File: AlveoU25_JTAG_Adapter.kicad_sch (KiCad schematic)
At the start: 11 parts, among them J1 Xilinx_JTAG, J3 OTHER, J4 OTHER, U1 Alveo_U25_Debug

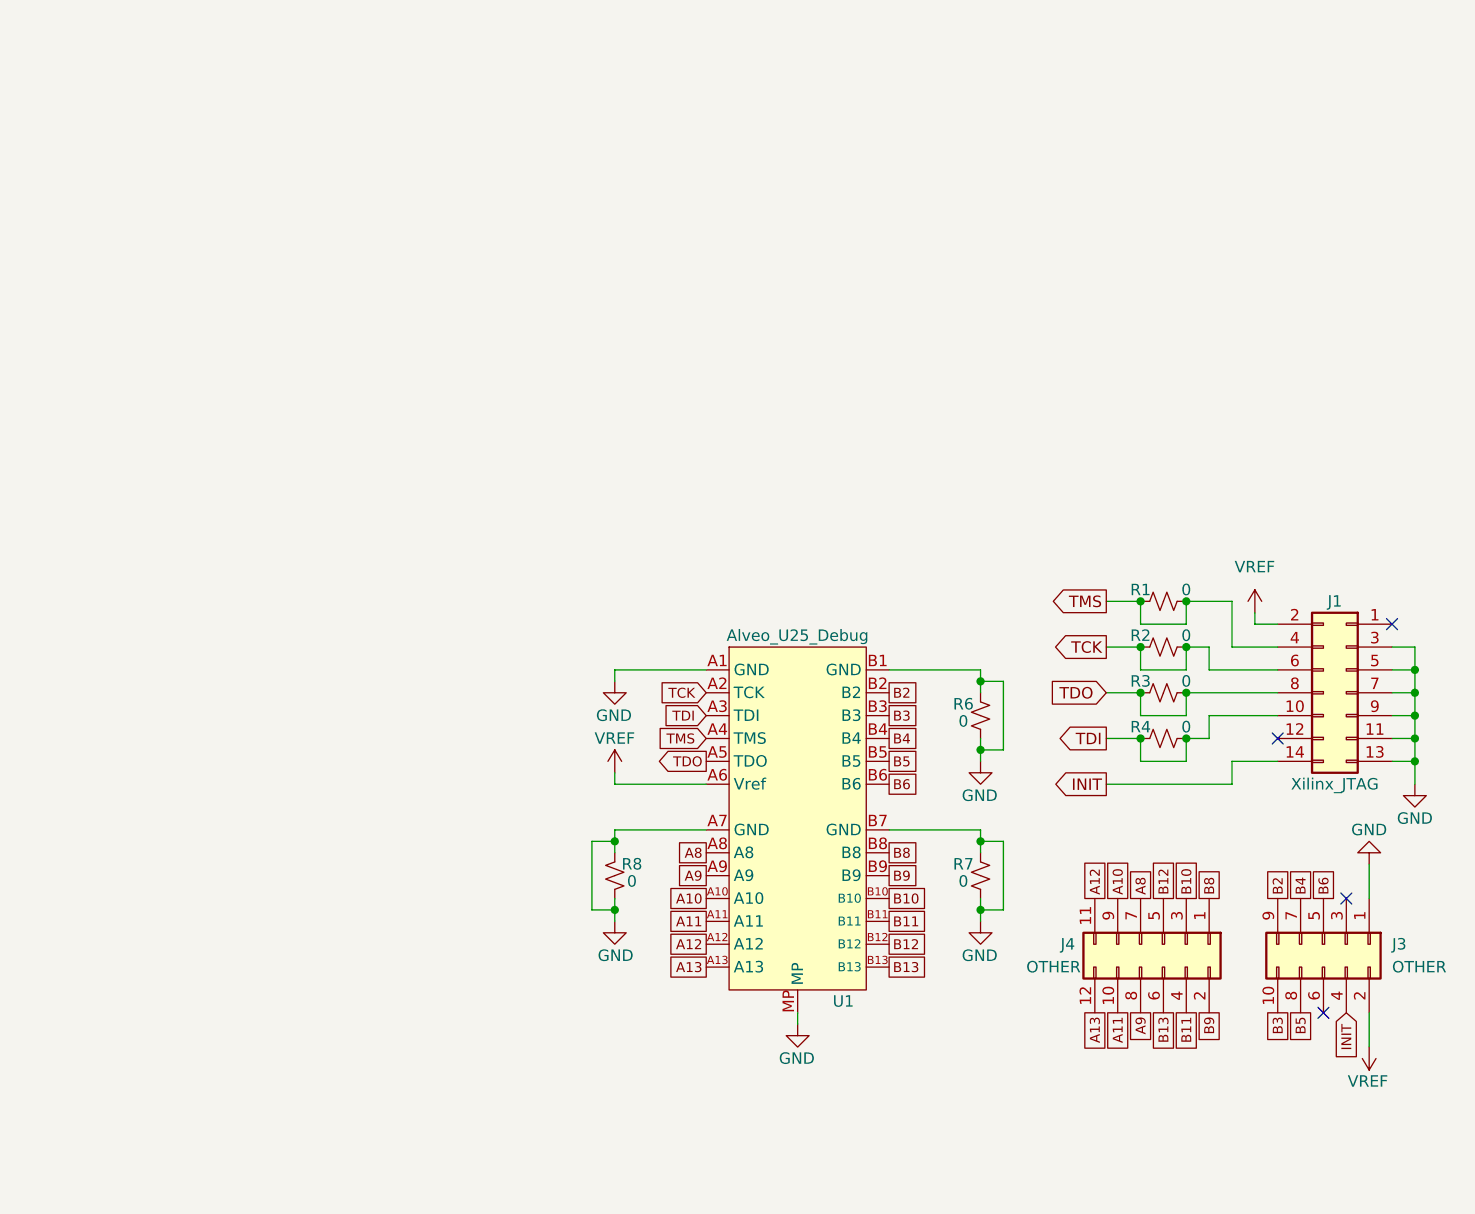
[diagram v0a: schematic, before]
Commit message: Second Revision
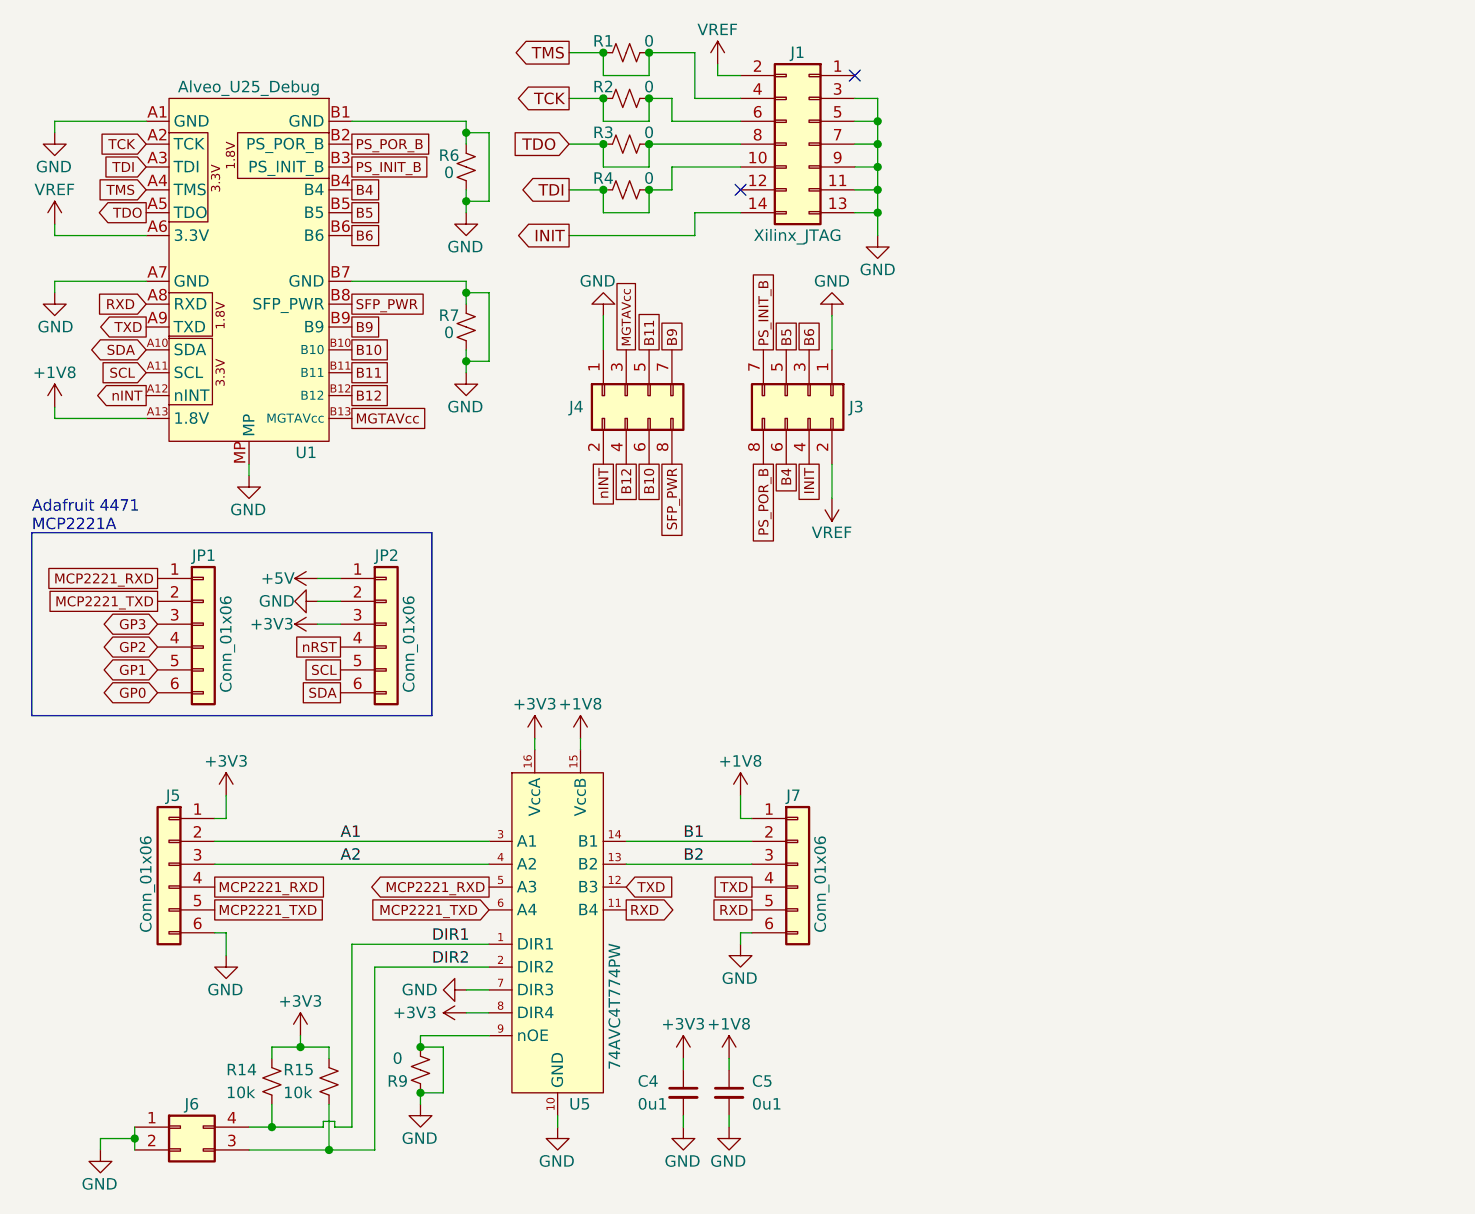
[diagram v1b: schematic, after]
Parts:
- removed J3: OTHER, Connector_PinHeader_2.54mm:PinHeader_2x05_P2.54mm_Vertical, symbol Connector_Generic:Conn_02x05_Odd_Even
- removed J4: OTHER, Connector_PinHeader_2.54mm:PinHeader_2x06_P2.54mm_Vertical, symbol Connector_Generic:Conn_02x06_Odd_Even
- removed R8: 0, Resistor_SMD:R_0603_1608Metric_Pad0.98x0.95mm_HandSolder, symbol Device:R_Small_US
- added C4, C5: 0u1, Capacitor_SMD:C_0603_1608Metric_Pad1.08x0.95mm_HandSolder, symbol Device:C_Small
- added J3, J4: Conn_02x04_Odd_Even, Connector_PinSocket_2.54mm:PinSocket_2x04_P2.54mm_Vertical, symbol Connector_Generic:Conn_02x04_Odd_Even
- added J5, J7, JP1, JP2: Conn_01x06, Connector_PinSocket_2.54mm:PinSocket_1x06_P2.54mm_Vertical, symbol Connector_Generic:Conn_01x06
- added J6: Conn_02x02_Counter_Clockwise, Connector_PinSocket_2.54mm:PinSocket_2x02_P2.54mm_Vertical, symbol Connector_Generic:Conn_02x02_Counter_Clockwise
- added R14, R15: 10k, Resistor_SMD:R_0603_1608Metric_Pad0.98x0.95mm_HandSolder, symbol Device:R_Small_US
- added R9: 0, Resistor_SMD:R_0603_1608Metric_Pad0.98x0.95mm_HandSolder, symbol Device:R_Small_US
- added U5: 74AVC4T774PW, Package_SO:TSSOP-16_4.4x5mm_P0.65mm, symbol 74AVC4T774PW:74AVC4T774PW
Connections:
- net +VREF: now also J3.2 (Pin_2)
- net B10: now also J4.6 (Pin_6)
- net B11: now also J4.5 (Pin_5)
- net B12: now also J4.4 (Pin_4)
- net B2: now also J7.3 (Pin_3), U5.13 (B2); no longer U1.B2
- net B4: now also J3.6 (Pin_6)
- net B5: now also J3.5 (Pin_5)
- net B6: now also J3.3 (Pin_3)
- net B9: now also J4.7 (Pin_7)
- net GND: now also C4.2, C5.2, J3.1 (Pin_1), J4.1 (Pin_1), J5.6 (Pin_6), J6.1 (Pin_1), J6.2 (Pin_2), J7.6 (Pin_6), JP2.2 (Pin_2), R9.1, R9.2, U5.10 (GND), U5.7 (DIR3), U5.9 (nOE)
- net INIT: now also J3.4 (Pin_4)
- net A10 renamed SDA
- net SDA: now also JP2.6 (Pin_6)
- net A11 renamed SCL
- net SCL: now also JP2.5 (Pin_5)
- net A12 renamed nINT
- net nINT: now also J4.2 (Pin_2)
- net A13 renamed +1V8
- net +1V8: now also C5.1, J7.1 (Pin_1), U5.15 (VccB)
- net A8 renamed RXD
- net RXD: now also J7.5 (Pin_5), U5.11 (B4)
- net A9 renamed TXD
- net TXD: now also J7.4 (Pin_4), U5.12 (B3)
- net B13 renamed MGTAVcc
- net MGTAVcc: now also J4.3 (Pin_3)
- net B3 renamed PS_INIT_B
- net PS_INIT_B: now also J3.7 (Pin_7)
- net B8 renamed SFP_PWR
- net SFP_PWR: now also J4.8 (Pin_8)
- new net +3V3: C4.1, J5.1 (Pin_1), JP2.3 (Pin_3), R14.1, R15.1, U5.16 (VccA), U5.8 (DIR4)
- new net +5V: JP2.1 (Pin_1)
- new net A1: J5.2 (Pin_2), U5.3 (A1)
- new net A2: J5.3 (Pin_3), U5.4 (A2)
- new net B1: J7.2 (Pin_2), U5.14 (B1)
- new net DIR1: J6.4 (Pin_4), R14.2, U5.1 (DIR1)
- new net DIR2: J6.3 (Pin_3), R15.2, U5.2 (DIR2)
- new net GP0: JP1.6 (Pin_6)
- new net GP1: JP1.5 (Pin_5)
- new net GP2: JP1.4 (Pin_4)
- new net GP3: JP1.3 (Pin_3)
- new net MCP2221_RXD: J5.4 (Pin_4), JP1.1 (Pin_1), U5.5 (A3)
- new net MCP2221_TXD: J5.5 (Pin_5), JP1.2 (Pin_2), U5.6 (A4)
- new net PS_POR_B: J3.8 (Pin_8), U1.B2 (PS_POR_B)
- new net nRST: JP2.4 (Pin_4)
- no-connect marks 4 -> 2
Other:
- note added: "Adafruit 4471 MCP2221A"
- moved on the sheet: J1, R1, R2, R3, R4, R6, R7
